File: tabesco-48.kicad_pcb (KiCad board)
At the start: 2 copper layers, 192.5 x 118.4 mm, 98 parts, among them SW1 SW_Push, U1 ProMicro

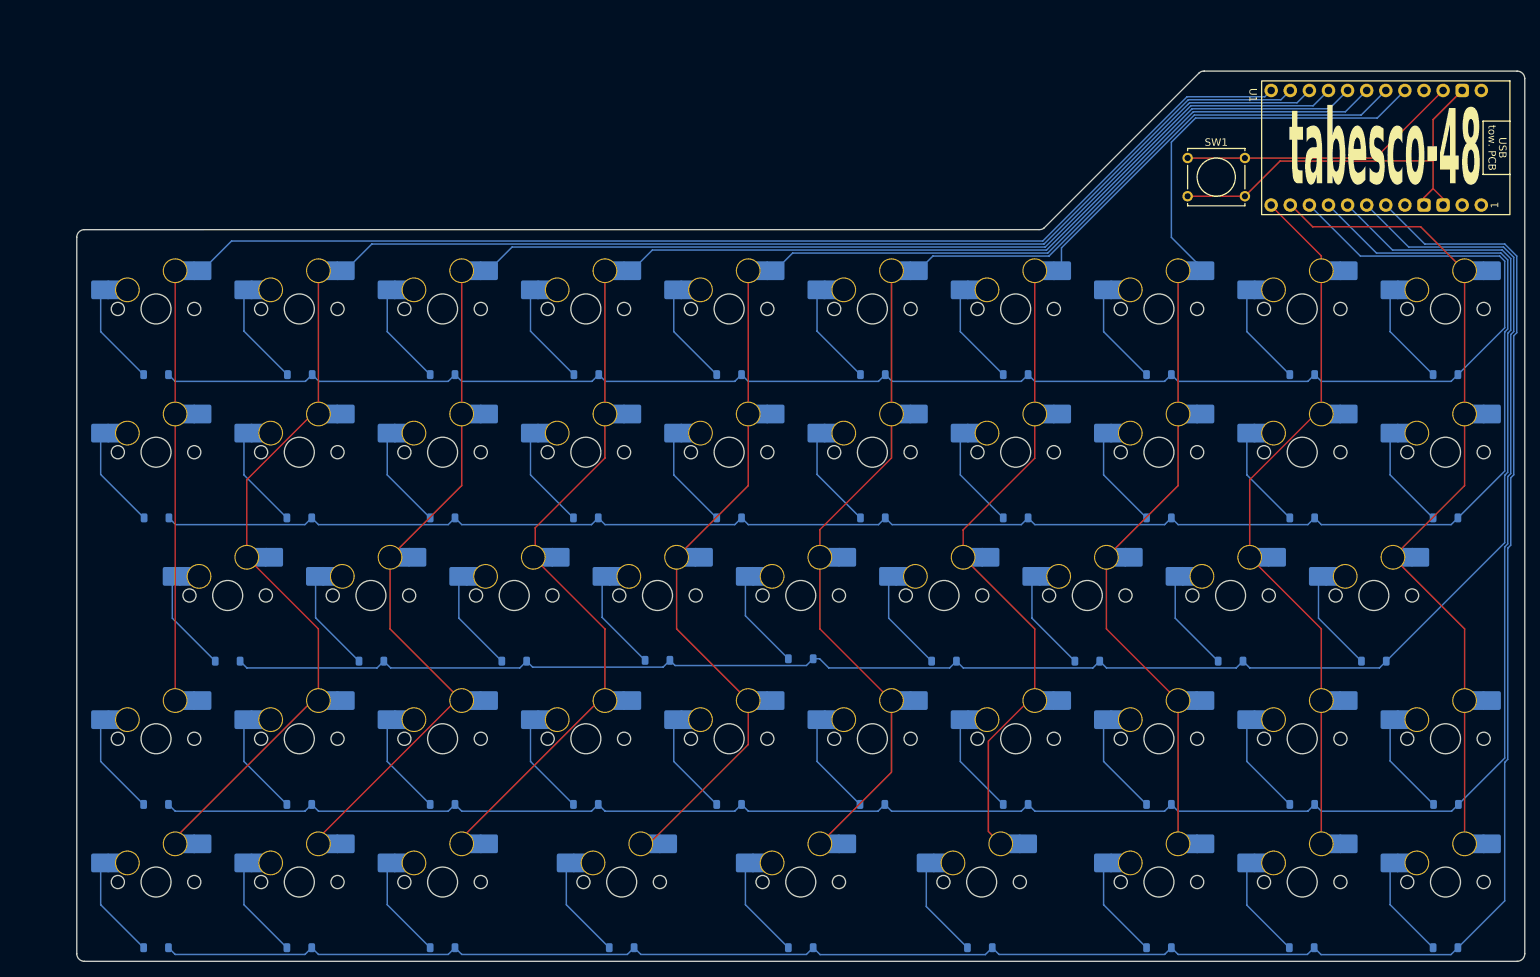
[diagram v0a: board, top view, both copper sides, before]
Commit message: created tabesco-31
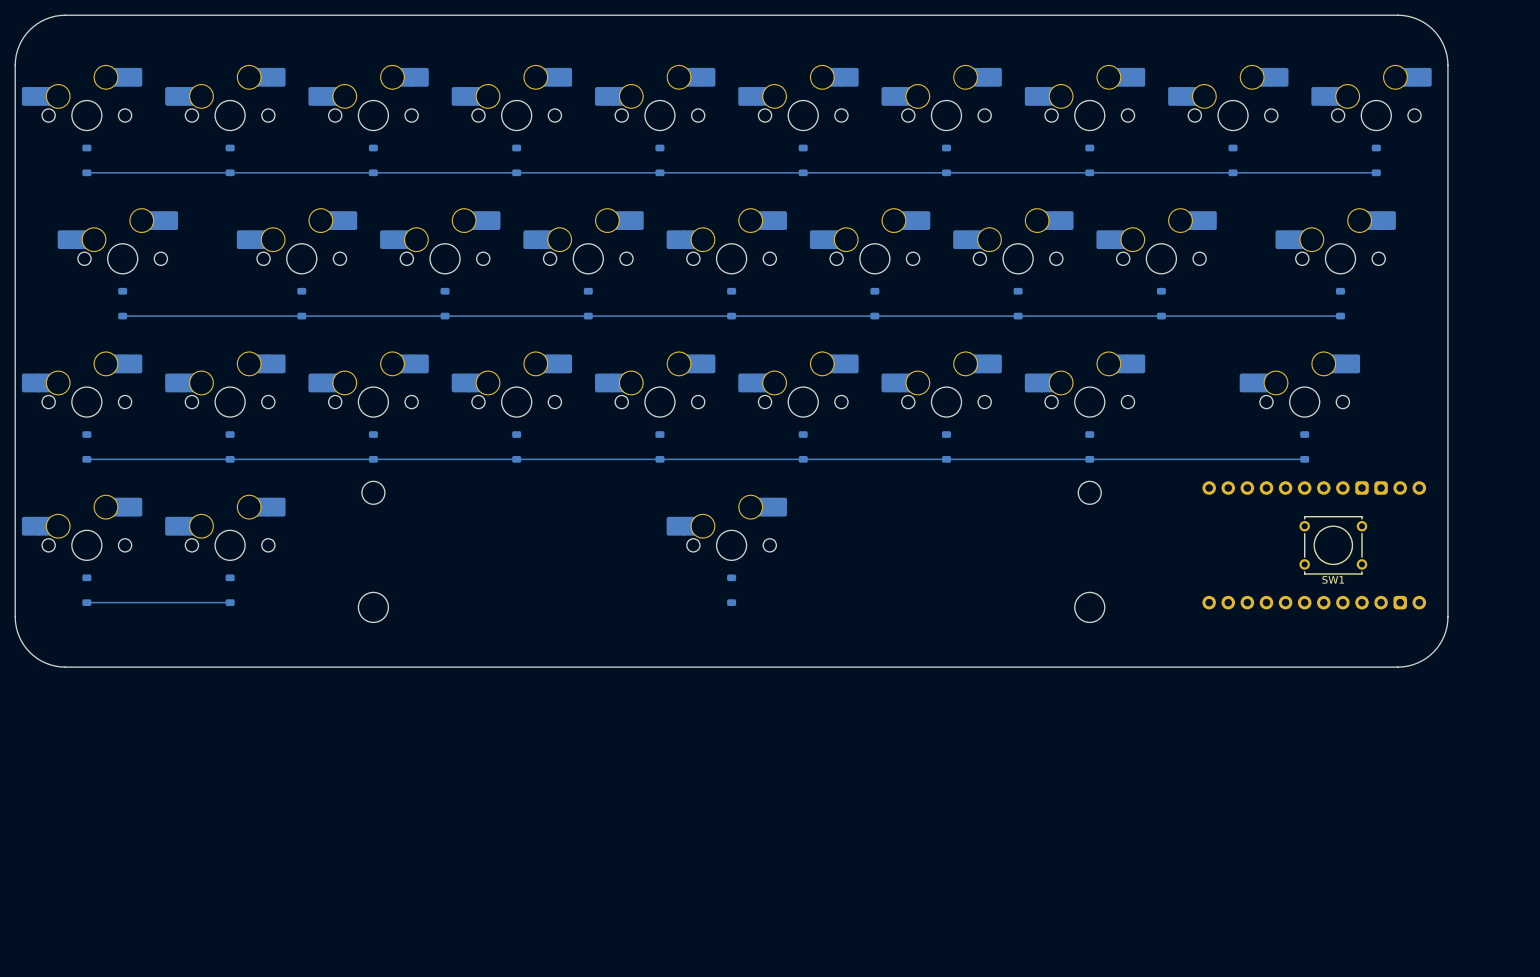
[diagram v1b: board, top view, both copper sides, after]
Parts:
- removed D32, D33, D34, D35, D36, D37, D38, D39, D40, D41, D42, D43, D44, D45, D46, D47, D48: D_Small, Diode_SMD:D_SOD-123
- removed MX32, MX33, MX34, MX35, MX36, MX37, MX38, MX39, MX40, MX41, MX42, MX43, MX44, MX45, MX46, MX47, MX48: MX_SW_HS, marbastlib-mx:SW_MX_HS_CPG151101S11_1u
- added REF**: STAB_MX_6u, marbastlib-mx:STAB_MX_6u, F.Cu at (146.0, 89.3)
- U1: moved to B.Cu
- moved D1 182.9 mm to (60.3, 38.2), turned to 90 degrees
- moved MX1 182.5 mm to (60.3, 32.2)
- moved D11 178.2 mm to (65.0, 57.2), turned to 90 degrees
- moved MX11 177.8 mm to (65.0, 51.2)
- moved D10 164.7 mm to (231.7, 38.2), turned to 90 degrees
- moved MX10 164.3 mm to (231.7, 32.2)
- moved D30 164.1 mm to (79.3, 95.3), turned to 90 degrees
- moved MX30 163.6 mm to (79.3, 89.3)
- moved MX21 154.2 mm to (79.3, 70.3)
- moved D2 145.4 mm to (79.3, 38.2), turned to 90 degrees
- moved MX2 144.8 mm to (79.3, 32.2)
- moved D19 141.3 mm to (227.0, 57.2), turned to 90 degrees
- moved MX19 140.8 mm to (227.0, 51.2)
- moved D12 136.0 mm to (88.8, 57.2), turned to 90 degrees
- moved MX12 135.5 mm to (88.8, 51.2)
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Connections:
- D20 pad 1: /row1 -> /row2
- D29 pad 1: /row2 -> /row3
- MX20 pad 2: /col9 -> /col0
- MX21 pad 2: /col0 -> /col1
- MX22 pad 2: /col1 -> /col2
- MX23 pad 2: /col2 -> /col3
- MX24 pad 2: /col3 -> /col4
- MX25 pad 2: /col4 -> /col5
- MX26 pad 2: /col5 -> /col6
- MX27 pad 2: /col6 -> /col7
- MX28 pad 2: /col7 -> /col8
- MX29 pad 2: /col8 -> /col0
- MX30 pad 2: /col0 -> /col1
- MX31 pad 2: /col1 -> /col7
- U1 pad 5: /col_tmo -> unconnected-(U1-D1-Pad5)
- U1 pad 6: /row4 -> unconnected-(U1-D0-Pad6)
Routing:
- net /row4: track 292.9 -> 0.00 mm
- net /row3: track 276.5 -> 19.0 mm
- net /col8: track 228.5 -> 0.00 mm
- net /col7: track 211.5 -> 0.00 mm
- net /col9: track 209.3 -> 0.00 mm
- net /col6: track 195.2 -> 0.00 mm
- net /col5: track 176.7 -> 0.00 mm
- net /col4: track 157.6 -> 0.00 mm
- net /col3: track 142.6 -> 0.00 mm
- net /col2: track 136.9 -> 0.00 mm
- net /col0: track 111.3 -> 0.00 mm
- net /col1: track 96.1 -> 0.00 mm
- net /row2: track 243.4 -> 161.9 mm
- net /row1: track 242.0 -> 161.9 mm
- net GND: track 54.7 -> 0.00 mm
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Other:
- board size 192.5 x 118.4 mm -> 190.5 x 86.7 mm
- board text removed: "tabesco-48"
